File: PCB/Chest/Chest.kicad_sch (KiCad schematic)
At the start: 35 parts, among them J1 Reset, J2 TF_PUSH, J3 TC2030-USB-NL-DS, J4 SPK, J5 USB-C-Socket-H, J7 SPK, U1 MAX98357A, U2 ESP32-S3-MINI-1, U2 MAX98357A, U5 MD8942

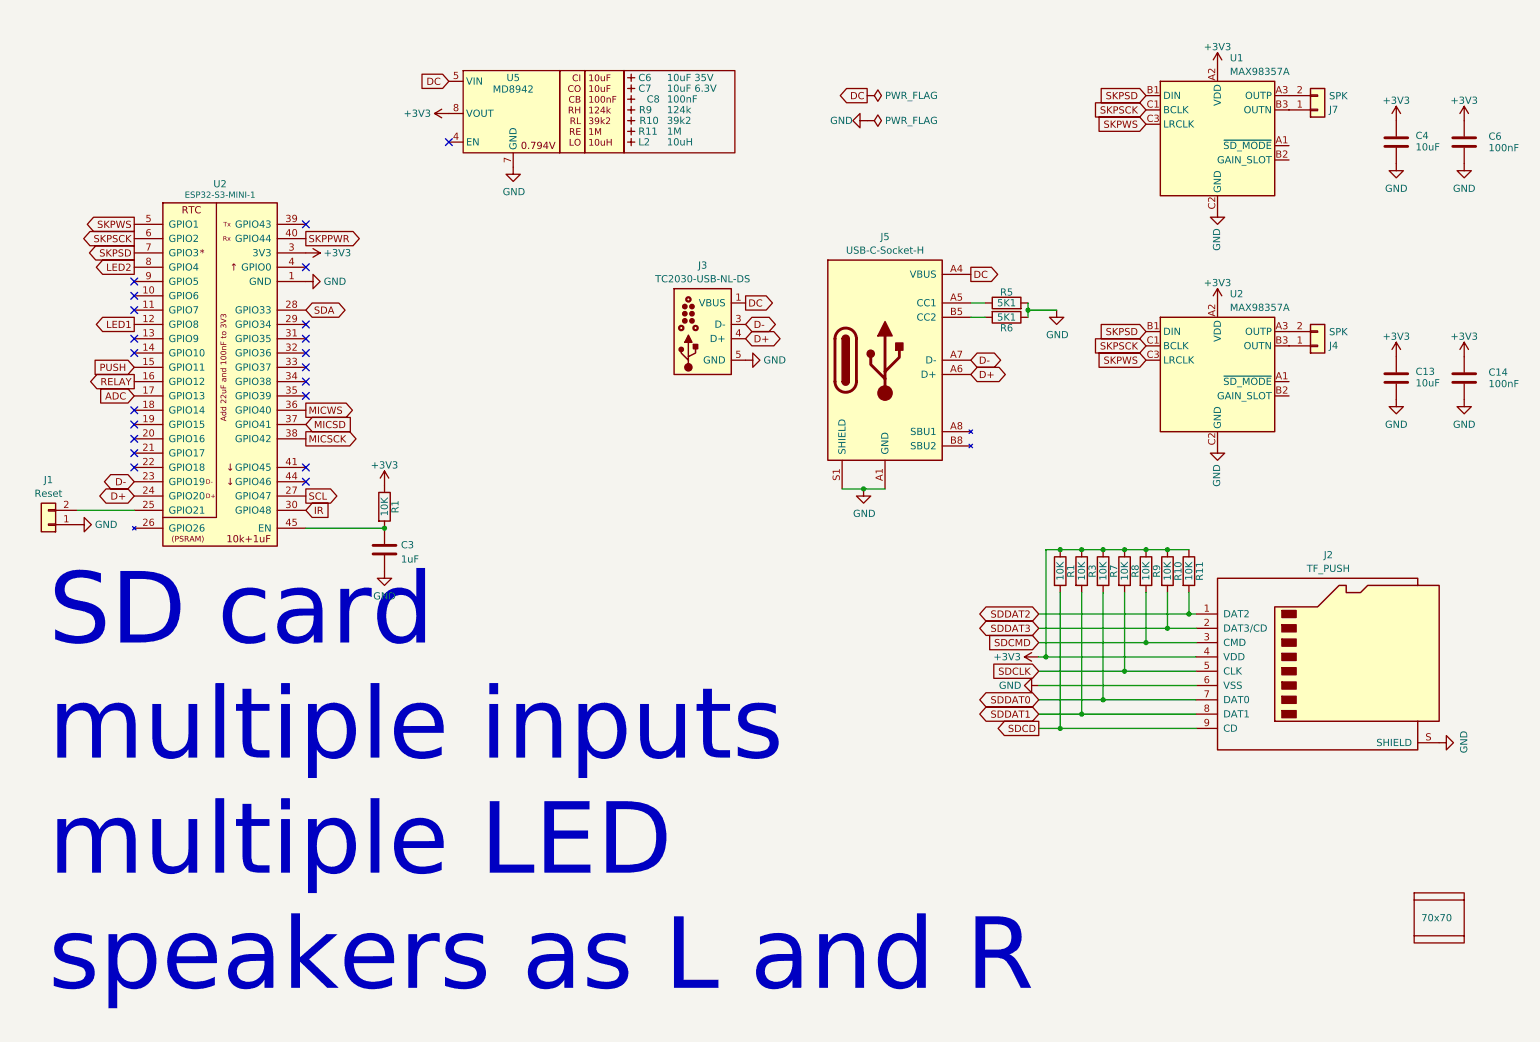
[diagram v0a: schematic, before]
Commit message: Started Chest board
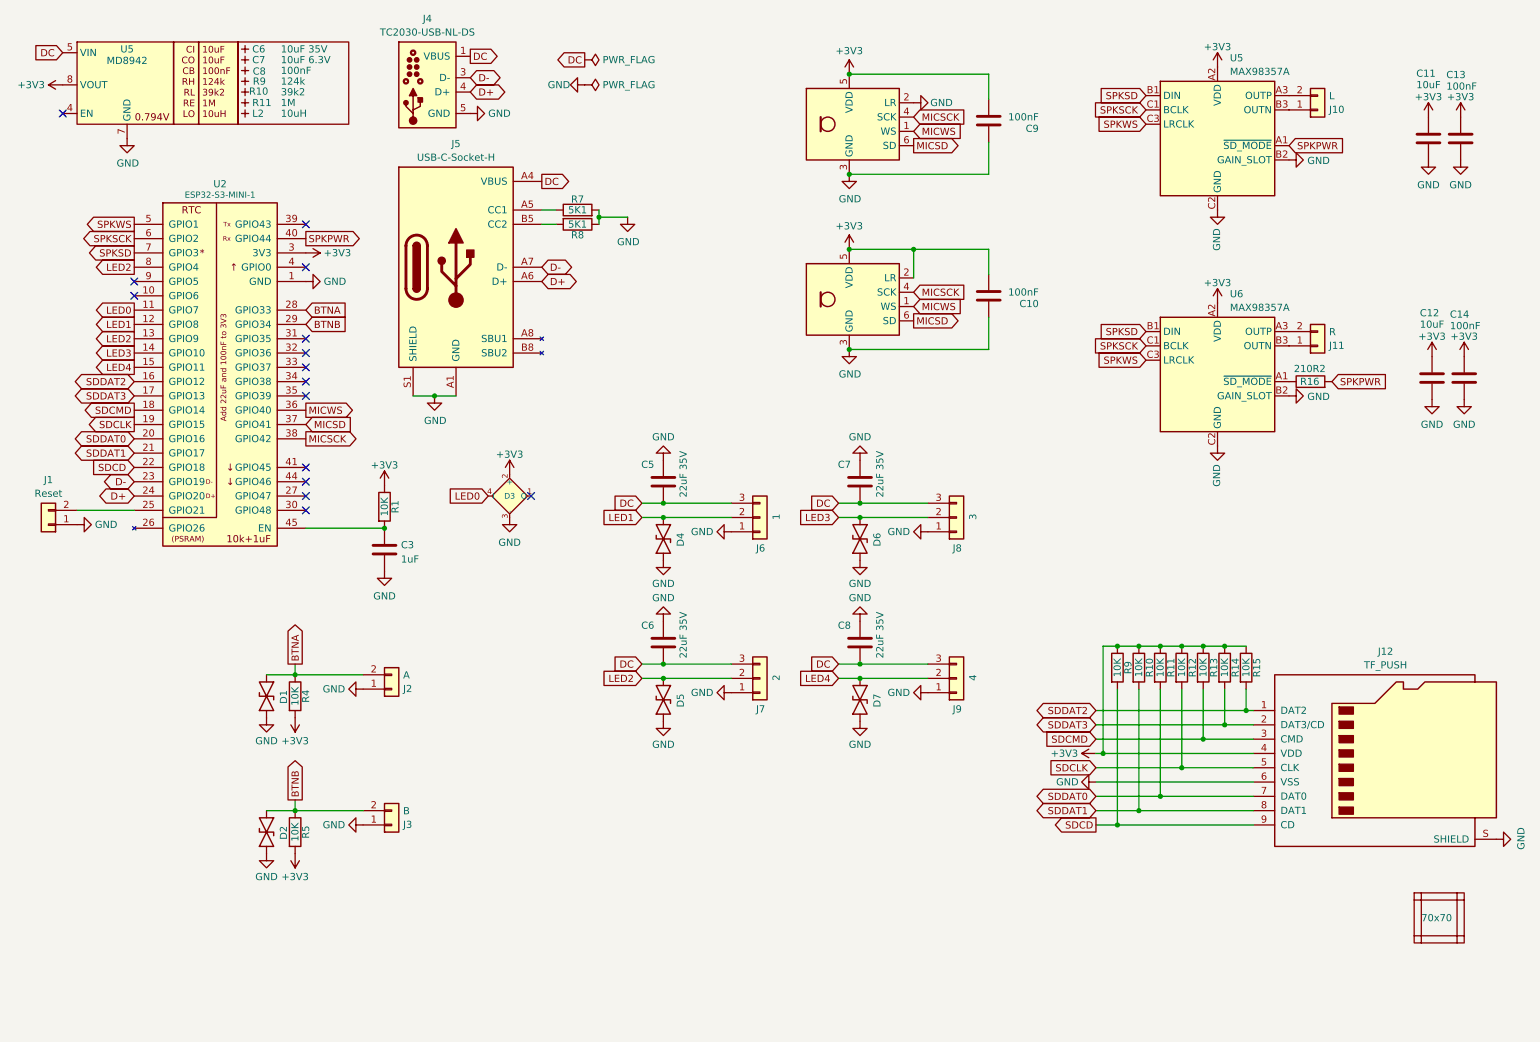
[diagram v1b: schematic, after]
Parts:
- removed C4: 10uF, RevK:C_0402, symbol Device:C
- added C10, C13, C9: 100nF, RevK:C_0402, symbol Device:C
- added C11: 10uF, RevK:C_0402, symbol Device:C
- added C5, C7, C8: 22uF 35V, RevK:C_1210, symbol Device:C
- added D1, D2, D4, D5, D6, D7: ~, RevK:DFN1006-2L, symbol RevK:ES05D1MC10
- added D3: XL-1010RGBC-WS2812B, RevK:SMD1010, symbol RevK:WS2812B-1mm
- added J2: A, RevK:WAGO-2060-452-998-404, symbol Connector_Generic:Conn_01x02
- added J3: B, RevK:WAGO-2060-452-998-404, symbol Connector_Generic:Conn_01x02
- added J6: 1, RevK:WAGO-2060-453-998-404, symbol Connector_Generic:Conn_01x03
- added J7: 2, RevK:WAGO-2060-453-998-404, symbol Connector_Generic:Conn_01x03
- added J8: 3, RevK:WAGO-2060-453-998-404, symbol Connector_Generic:Conn_01x03
- added J9: 4, RevK:WAGO-2060-453-998-404, symbol Connector_Generic:Conn_01x03
- added R16: 210R2, RevK:R_0402, symbol Device:R
- added R4, R5: 10K, RevK:R_0402, symbol Device:R
- added U3: L, RevK:ICS43434_MEMS_Mic_Open, symbol RevK:ICS43434_MEMS_Mic
- added U4: R, RevK:ICS43434_MEMS_Mic_Open, symbol RevK:ICS43434_MEMS_Mic
- added V3, V4: ~, RevK:VCUT70N, symbol RevK:VCUT
- C6: value 100nF -> 22uF 35V; footprint RevK:C_0402 -> RevK:C_1210
- J10: renamed from J7; value SPK -> L
- J11: renamed from J4; value SPK -> R
- renumbered C13 to C12, J2 to J12, J3 to J4, R3 to R10, R7 to R11, R8 to R12, R9 to R13, R10 to R14, R11 to R15, R5 to R7, R6 to R8, R1 to R9, U1 to U5, U2 to U6
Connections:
- net ADC is gone; now on net SDDAT3: U2.17 (GPIO13)
- net RELAY is gone; now on net SDDAT2: U2.16 (GPIO12)
- net SKPPWR is gone; now on net SPKPWR: U2.40 (GPIO44)
- net +3V3: now also C10.2, C11.1, C13.1, C9.2, D3.2 (+), R4.2, R5.2, U3.5 (VDD), U4.2 (LR), U4.5 (VDD); no longer C6.1
- net DC: now also C6.2, C5.2, C7.2, C8.2, J6.3 (Pin_3), J7.3 (Pin_3), J8.3 (Pin_3), J9.3 (Pin_3)
- net GND: now also C6.1, U5.B2 (GAIN_SLOT), U6.B2 (GAIN_SLOT), C10.1, C11.2, C13.2, C5.1, C7.1, C8.1, C9.1, D1.2, D2.2, D3.3 (-), D4.2, D5.2, D6.2, D7.2, J2.1 (Pin_1), J3.1 (Pin_1), J6.1 (Pin_1), J7.1 (Pin_1), J8.1 (Pin_1), J9.1 (Pin_1), U3.2 (LR), U3.3 (GND), U4.3 (GND); no longer C6.2
- net LED1: now also D4.1, J6.2 (Pin_2)
- net LED2: now also U2.13 (GPIO9), D5.1, J7.2 (Pin_2)
- net MICSCK: now also U3.4 (SCK), U4.4 (SCK)
- net MICSD: now also U3.6 (SD), U4.6 (SD)
- net MICWS: now also U3.1 (WS), U4.1 (WS)
- net SDCD: now also U2.22 (GPIO18)
- net SDCLK: now also U2.19 (GPIO15)
- net SDCMD: now also U2.18 (GPIO14)
- net SDDAT0: now also U2.20 (GPIO16)
- net SDDAT1: now also U2.21 (GPIO17)
- net LED0: now reaches U2.11 (GPIO7)
- net LED0: now also D3.4 (I)
- net LED3: now reaches U2.14 (GPIO10)
- net LED3: now also D6.1, J8.2 (Pin_2)
- net BTNB: now reaches U2.29 (GPIO34)
- net BTNB: now also D2.1, J3.2 (Pin_2), R5.1
- net SPKPWR: now reaches U5.A1 (~{SD_MODE})
- net SPKPWR: now also R16.2
- net at U6.A1 (~{SD_MODE}): now also R16.1
- net IR: no longer names the net of U2.30 (GPIO48)
- net PUSH renamed LED4
- net LED4: now also D7.1, J9.2 (Pin_2)
- net SCL: no longer names the net of U2.27 (GPIO47)
- net SDA renamed BTNA
- net BTNA: now also D1.1, J2.2 (Pin_2), R4.1
- net SKPSCK renamed SPKSCK
- net SKPSD renamed SPKSD
- net SKPWS renamed SPKWS
- no-connect marks 21 -> 15
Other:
- note removed: "SD card multiple inputs multiple LED speakers as L and R"
- moved on the sheet: C12, C6, C7, C8, J12, J4, J5, L2, R10, R11, R12, R13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

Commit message: Tidy
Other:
- title: LED driver -> IronMan Chest
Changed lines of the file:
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@@
 	(paper "A4")
 	(title_block
-		(title "LED driver")
+		(title "IronMan Chest")
 		(rev "1")
 		(comment 1 "@TheRealRevK")
